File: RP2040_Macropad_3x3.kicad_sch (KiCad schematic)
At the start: 7 parts, among them U1 RP2040, U2 SSD1306_128x32

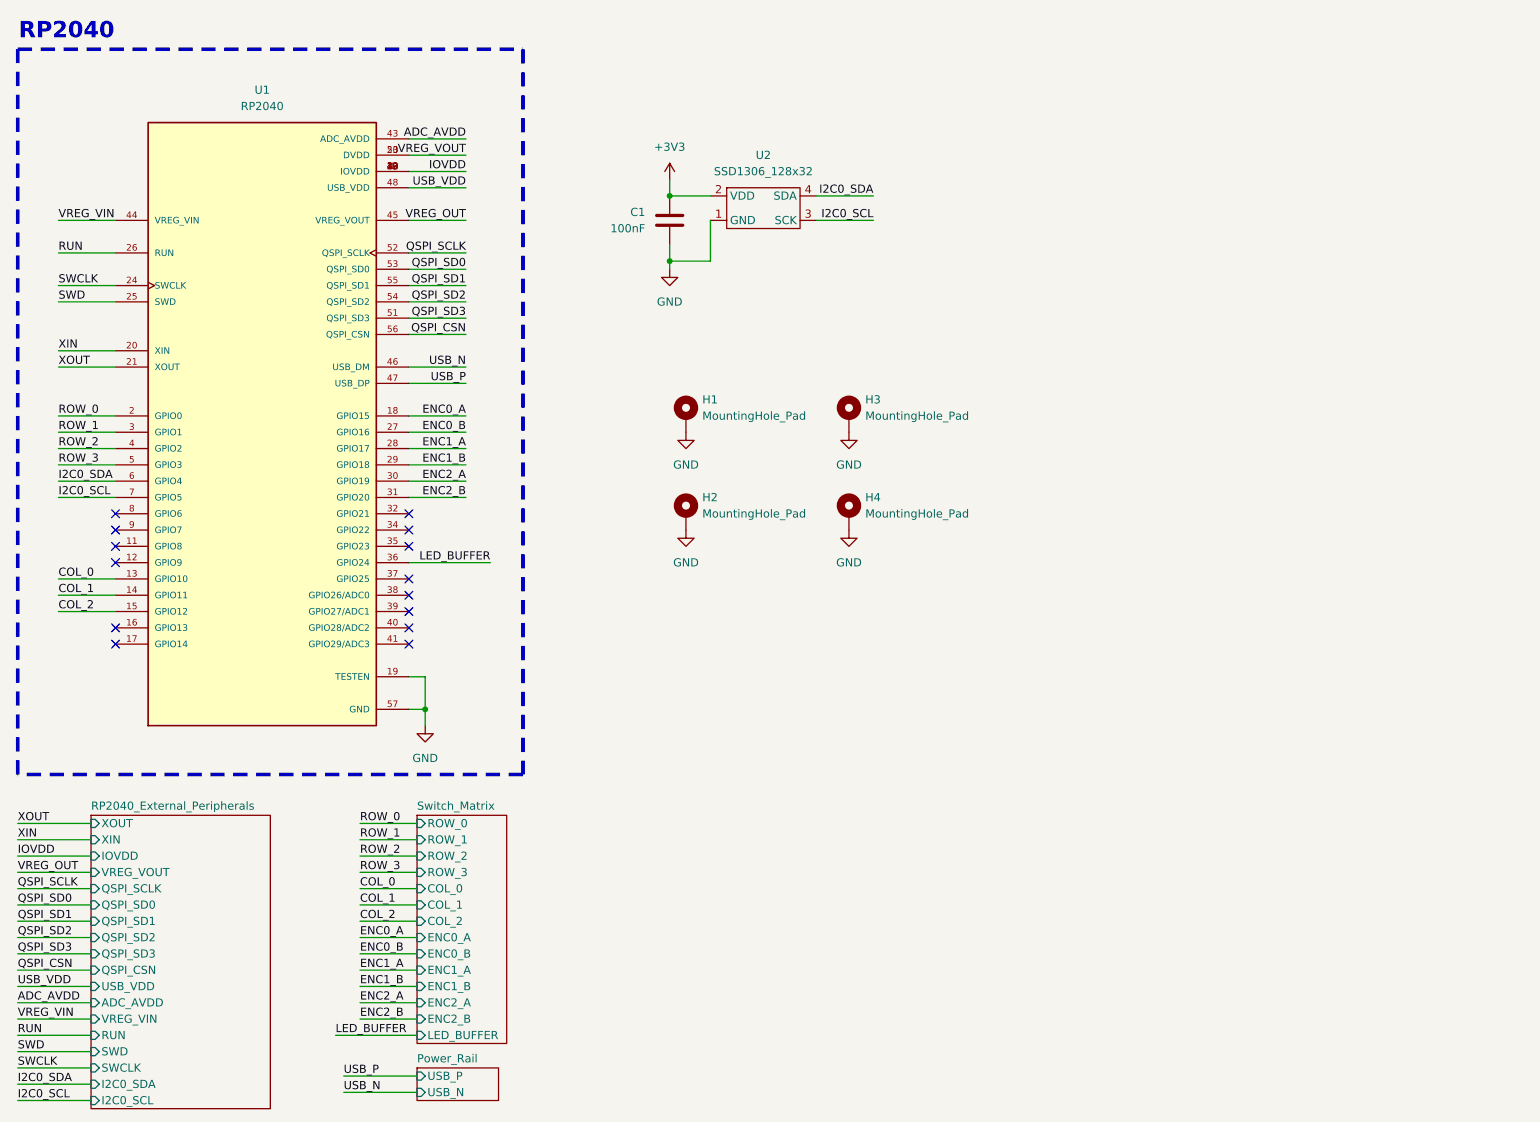
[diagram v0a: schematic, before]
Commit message: Schematic Clean Up
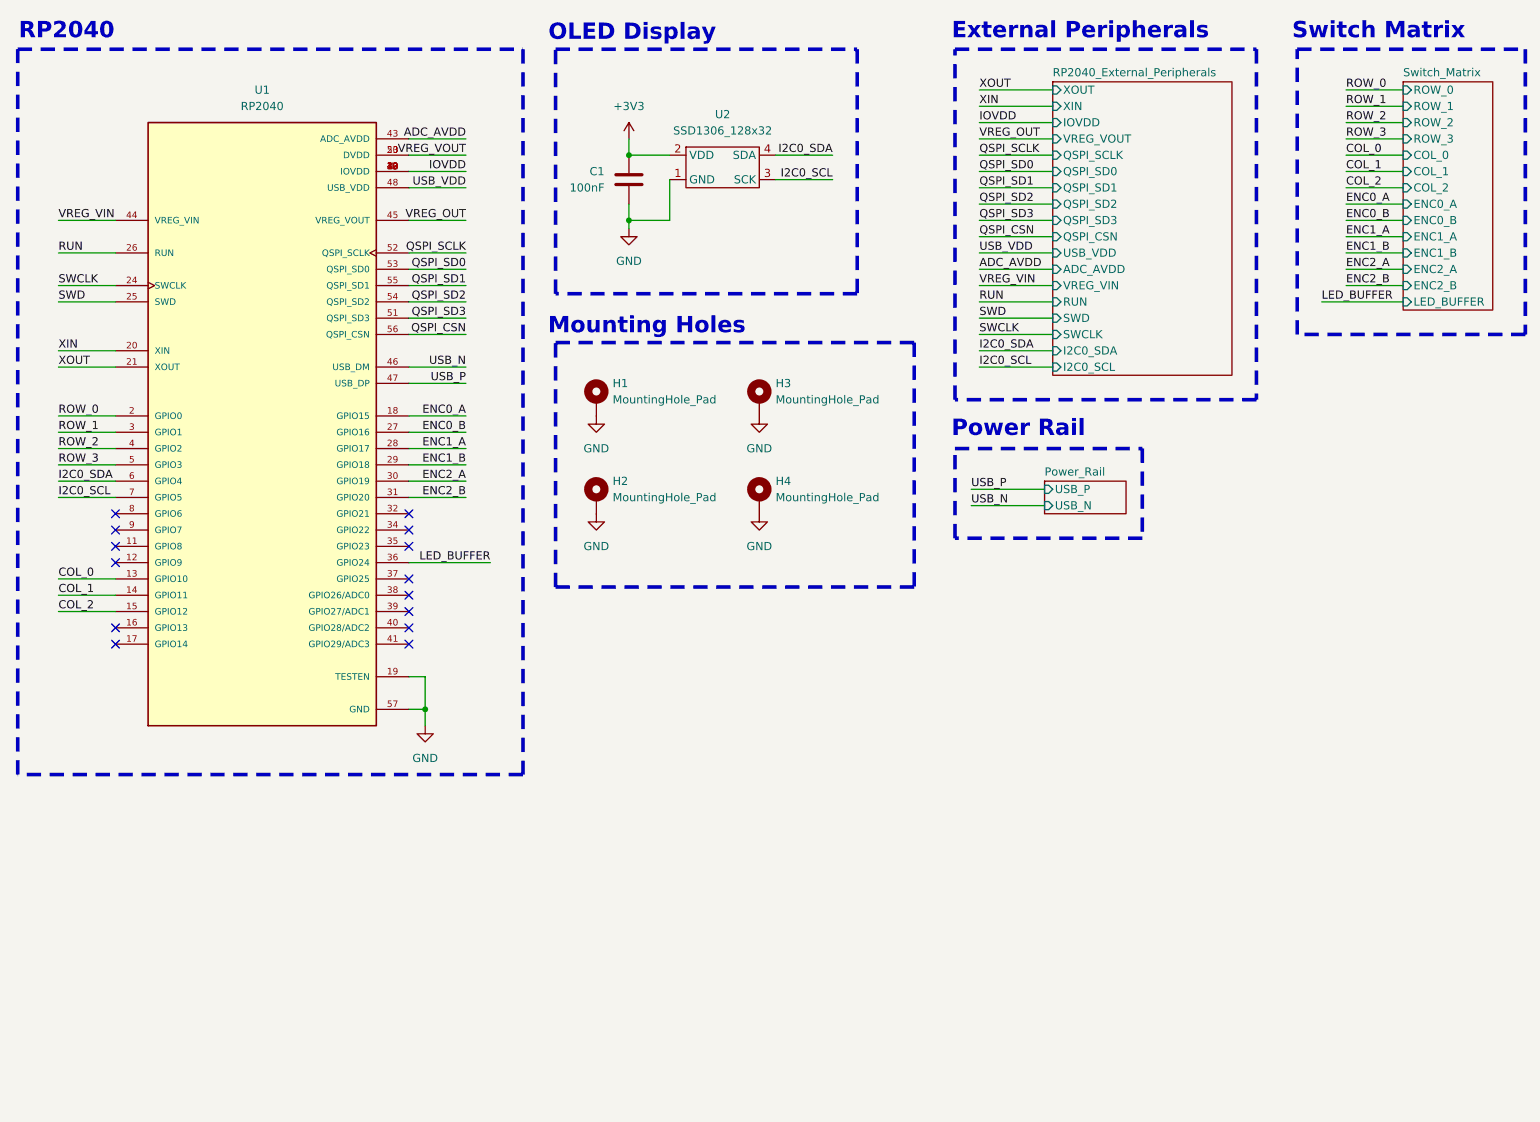
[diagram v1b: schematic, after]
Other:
- note added: "External Peripherals"
- note added: "Mounting Holes"
- note added: "OLED Display"
- note added: "Power Rail"
- note added: "Switch Matrix"
- moved on the sheet: C1, H1, H2, H3, H4, U2
